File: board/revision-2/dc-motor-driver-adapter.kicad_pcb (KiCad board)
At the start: 2 copper layers, 15.8 x 10 mm, 11 parts, among them J1 Conn_01x03, J2 Conn_01x03, U1 CH32V003J4M6

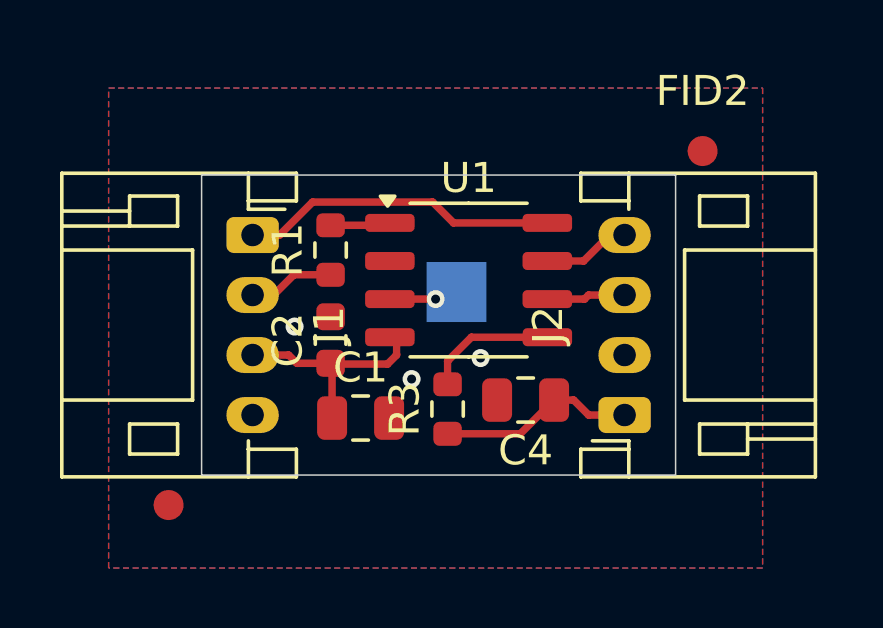
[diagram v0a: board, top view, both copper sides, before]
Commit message: Починаю працювати над I2C DAC.
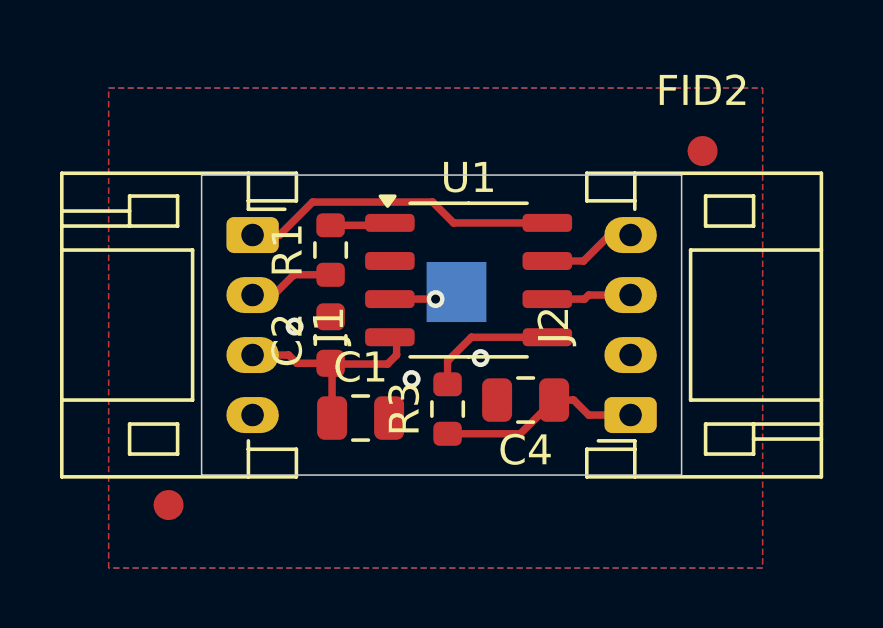
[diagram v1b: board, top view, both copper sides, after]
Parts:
- moved J2 0.20 mm to (171.6, 112.9)
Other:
- board size 15.8 x 10 mm -> 16 x 10 mm
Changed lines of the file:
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@@
 		(tags "SOP SO")
 		(property "Reference" "U1"
-			(at 0 -3.4 360)
+			(at 0 -3.4 0)
 			(layer "F.SilkS")
 			(effects
@@
 		)
 		(property "Value" "CH32V003J4M6"
-			(at 3.3 8.5 360)
+			(at 3.3 8.5 0)
 			(layer "F.Fab")
 			(hide yes)
@@
 		)
 		(fp_text user "${REFERENCE}"
-			(at 0 0 360)
+			(at 0 0 0)
 			(layer "F.Fab")
 			(effects
@@
 	(footprint "Connector_JST:JST_PH_S4B-PH-K_1x04_P2.00mm_Horizontal"
 		(layer "F.Cu")
-		(at 171.4 112.9 90)
+		(at 171.6 112.9 90)
 		(descr "JST PH series connector, S4B-PH-K (http://www.jst-mfg.com/product/pdf/eng/ePH.pdf), generated with kicad-footprint-generator")
 		(tags "connector JST PH top entry")
@@
 		(tags "capacitor")
 		(property "Reference" "C1"
-			(at 0 -1.679999 360)
+			(at 0 -1.679999 0)
 			(layer "F.SilkS")
 			(effects
@@
 		)
 		(property "Value" "10uF"
-			(at 0.6 3.599999 360)
+			(at 0.6 3.599999 0)
 			(layer "F.Fab")
 			(hide yes)
@@
 		)
 		(fp_text user "${REFERENCE}"
-			(at 0 -0.199999 360)
+			(at 0 -0.199999 0)
 			(layer "F.Fab")
 			(effects
@@
 		(tags "resistor")
 		(property "Reference" "R1"
-			(at 0 -1.43 270)
+			(at 0 -1.43 -90)
 			(layer "F.SilkS")
 			(effects
@@
 		)
 		(property "Value" "4.7k"
-			(at 0 1.43 270)
+			(at 0 1.43 -90)
 			(layer "F.Fab")
 			(hide yes)
@@
 		)
 		(fp_text user "${REFERENCE}"
-			(at 0 0 270)
+			(at 0 0 -90)
 			(layer "F.Fab")
 			(effects
@@
 		(tags "resistor")
 		(property "Reference" "R3"
-			(at 0 -1.43 270)
+			(at 0 -1.43 -90)
 			(layer "F.SilkS")
 			(effects
@@
 		)
 		(fp_text user "${REFERENCE}"
-			(at 0 0 270)
+			(at 0 0 -90)
 			(layer "F.Fab")
 			(effects
@@
 	)
 	(gr_circle
-		(center 171.4 108.9)
-		(end 171.85 108.9)
+		(center 171.6 108.9)
+		(end 172.05 108.9)
 		(stroke
 			(width 0.1)
@@
 	)
 	(gr_circle
-		(center 171.4 106.9)
-		(end 171.85 106.9)
+		(center 171.6 106.9)
+		(end 172.05 106.9)
 		(stroke
 			(width 0.1)
@@
 	)
 	(gr_circle
-		(center 171.4 110.9)
-		(end 171.85 110.9)
+		(center 171.6 110.9)
+		(end 172.05 110.9)
 		(stroke
 			(width 0.1)
@@
 	)
 	(gr_circle
-		(center 171.4 112.9)
-		(end 171.85 112.9)
+		(center 171.6 112.9)
+		(end 172.05 112.9)
 		(stroke
 			(width 0.1)
@@
 	(gr_rect
 		(start 157.3 104.9)
-		(end 173.1 114.9)
+		(end 173.3 114.9)
 		(stroke
 			(width 0.05)
@@
 		(layer "Dwgs.User")
 		(pts
-			(xy 157.3 104.9) (xy 173.1 104.9)
+			(xy 157.3 104.9) (xy 173.3 104.9)
 		)
 		(height -5)
-		(gr_text "15.8000 mm"
-			(at 165.2 98.75 0)
+		(gr_text "16.0000 mm"
+			(at 165.3 98.75 0)
 			(layer "Dwgs.User")
 			(effects
